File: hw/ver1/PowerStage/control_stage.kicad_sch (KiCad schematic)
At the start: 11 parts, among them J10 SWD Debug, J11 BMS_Serial, J8 FanConnector, P1 USB_C_Plug_USB2.0, SW2 I2C_Addr, U10 RP2040, U4 LM1117MP-3.3

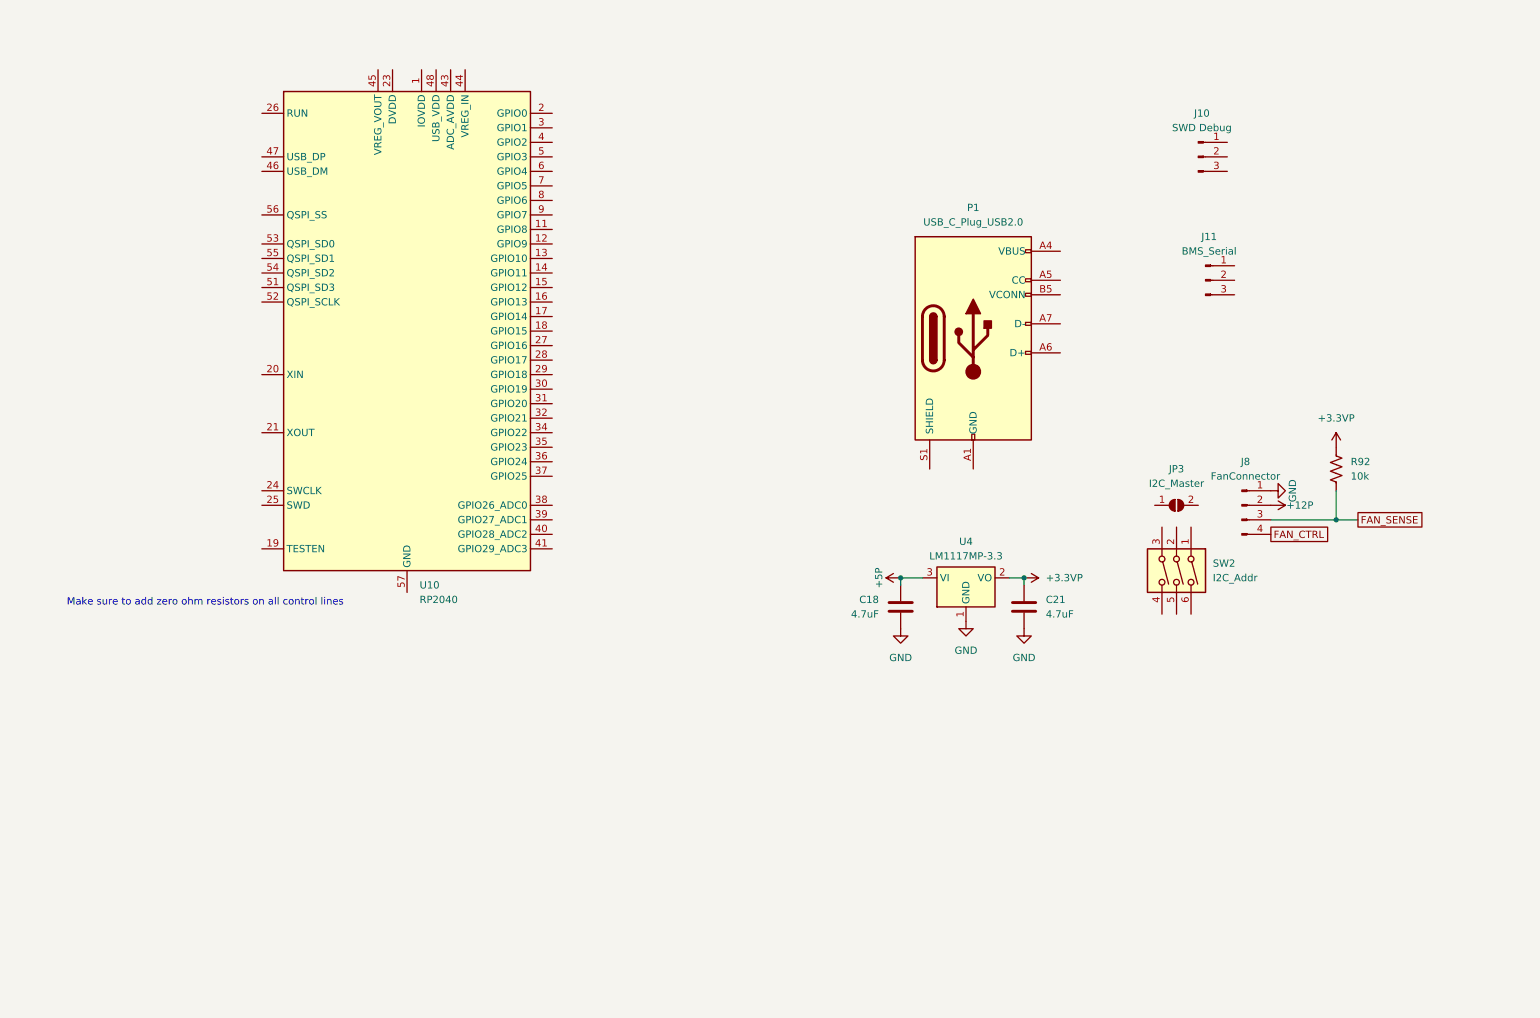
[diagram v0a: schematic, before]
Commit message: Sync this morning's effort
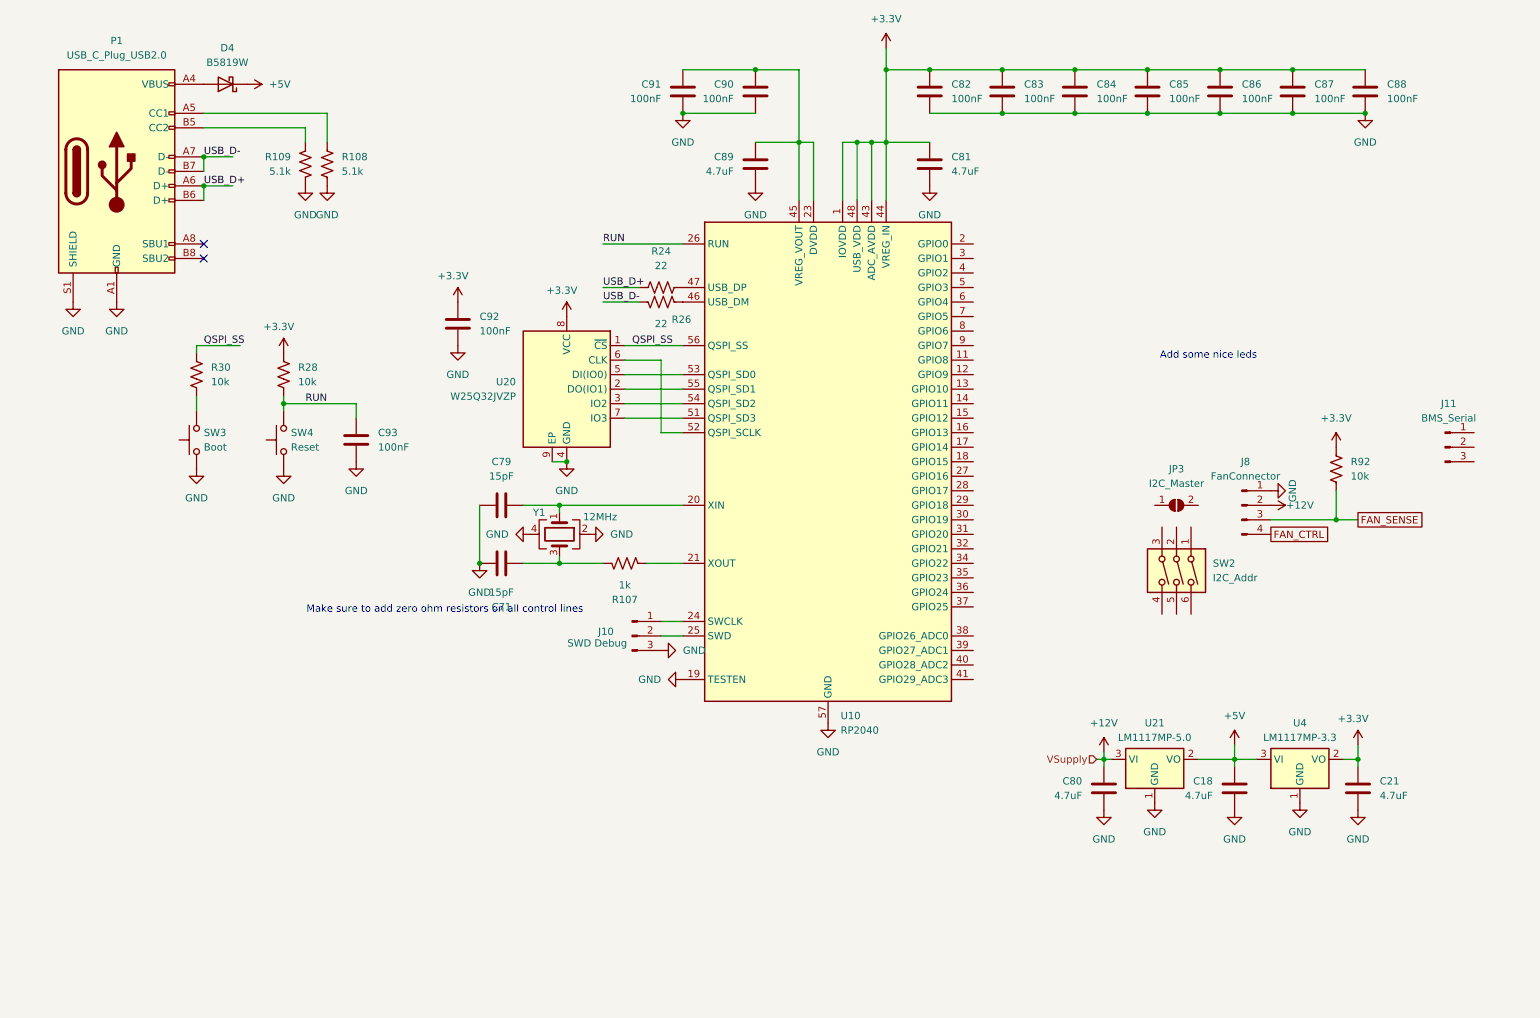
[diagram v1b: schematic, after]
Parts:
- added C71, C79: 15pF, Capacitor_SMD:C_0603_1608Metric, symbol Device:C
- added C80, C81, C89: 4.7uF, Capacitor_SMD:C_0603_1608Metric, symbol Device:C
- added C82, C83, C84, C85, C86, C87, C88, C90, C91, C92, C93: 100nF, Capacitor_SMD:C_0603_1608Metric, symbol Device:C
- added D4: B5819W, Diode_SMD:D_SOD-123, symbol Device:D_Schottky
- added R107: 1k, Resistor_SMD:R_0603_1608Metric, symbol Device:R_US
- added R108, R109: 5.1k, Resistor_SMD:R_0603_1608Metric, symbol Device:R_US
- added R24, R26: 22, Resistor_SMD:R_0603_1608Metric, symbol Device:R_US
- added R28, R30: 10k, Resistor_SMD:R_0603_1608Metric, symbol Device:R_US
- added SW3: Boot, symbol Switch:SW_Push
- added SW4: Reset, symbol Switch:SW_Push
- added U20: W25Q32JVZP, Package_SON:WSON-8-1EP_6x5mm_P1.27mm_EP3.4x4.3mm, symbol Memory_Flash:W25Q32JVZP
- added U21: LM1117MP-5.0, Package_TO_SOT_SMD:SOT-223-3_TabPin2, symbol Regulator_Linear:LM1117MP-5.0
- added Y1: 12MHz, Crystal:Crystal_SMD_3225-4Pin_3.2x2.5mm_HandSoldering, symbol Device:Crystal_GND24
- P1: symbol Connector:USB_C_Plug_USB2.0 -> Connector:USB_C_Receptacle_USB2.0_16P
- U4: LCSC C23984 -> C6186
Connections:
- net +3.3VP is gone; now on net +3.3V: C21.1, R92.2, U4.2 (VO)
- net GND: now also J10.3 (Pin_3), P1.A1 (GND), P1.A12 (GND), P1.B1 (GND), P1.B12 (GND), P1.S1 (SHIELD), U10.19 (TESTEN), U10.57 (GND), C71.1, C79.1, C80.2, C81.2, C82.2, C83.2, C84.2, C85.2, C86.2, C87.2, C88.2, C89.2, C90.2, C91.2, C92.2, C93.2, R108.1, R109.1, SW3.1, SW4.1, U20.4 (GND), U20.9 (EP), U21.1 (GND), Y1.2, Y1.4
- net +3.3V: now reaches U10.1 (IOVDD), U10.10 (IOVDD), U10.22 (IOVDD), U10.33 (IOVDD), U10.42 (IOVDD), U10.49 (IOVDD)
- net +3.3V: now also U10.43 (ADC_AVDD), U10.44 (VREG_IN), U10.48 (USB_VDD), C81.1, C82.1, C83.1, C84.1, C85.1, C86.1, C87.1, C88.1, C92.1, R28.2, U20.8 (VCC)
- net at U10.20 (XIN): now also C79.2, Y1.1
- net at U10.21 (XOUT): now also R107.2
- net at U10.23 (DVDD), U10.50 (DVDD): now also U10.45 (VREG_VOUT), C89.1, C90.1, C91.1
- net at U10.24 (SWCLK): now also J10.1 (Pin_1)
- net at U10.25 (SWD): now also J10.2 (Pin_2)
- net RUN: now reaches U10.26 (RUN)
- net RUN: now also C93.1, R28.1, SW4.2
- net at U10.46 (USB_DM): now also R26.1
- net at U10.47 (USB_DP): now also R24.1
- net at U10.51 (QSPI_SD3): now also U20.7 (IO3)
- net at U10.52 (QSPI_SCLK): now also U20.6 (CLK)
- net at U10.53 (QSPI_SD0): now also U20.5 (DI(IO0))
- net at U10.54 (QSPI_SD2): now also U20.3 (IO2)
- net at U10.55 (QSPI_SD1): now also U20.2 (DO(IO1))
- net QSPI_SS: now reaches U10.56 (QSPI_SS)
- net QSPI_SS: now also R30.2, U20.1 (~{CS})
- net at P1.A4 (VBUS), P1.A9 (VBUS), P1.B4 (VBUS)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: now also D4.2 (A)
- net at P1.A5 (CC1): now also R108.2
- net USB_D+: now reaches P1.A6 (D+)
- net USB_D+: now also P1.B6 (D+), R24.2
- net USB_D-: now reaches P1.A7 (D-)
- net USB_D-: now also P1.B7 (D-), R26.2
- net at P1.B5 (CC2): now also R109.2
- net +12P renamed +12V
- net +12V: now also C80.1, U21.3 (VI)
- net +5P renamed +5V
- net +5V: now also D4.1 (K), U21.2 (VO)
- new net: R30.1, SW3.2
- new net: C71.2, R107.1, Y1.3
- no-connect marks 0 -> 2
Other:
- note added: "Add some nice leds"
- moved on the sheet: C18, C21, J10, J11, U10, U4

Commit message: Sync tonight's effort
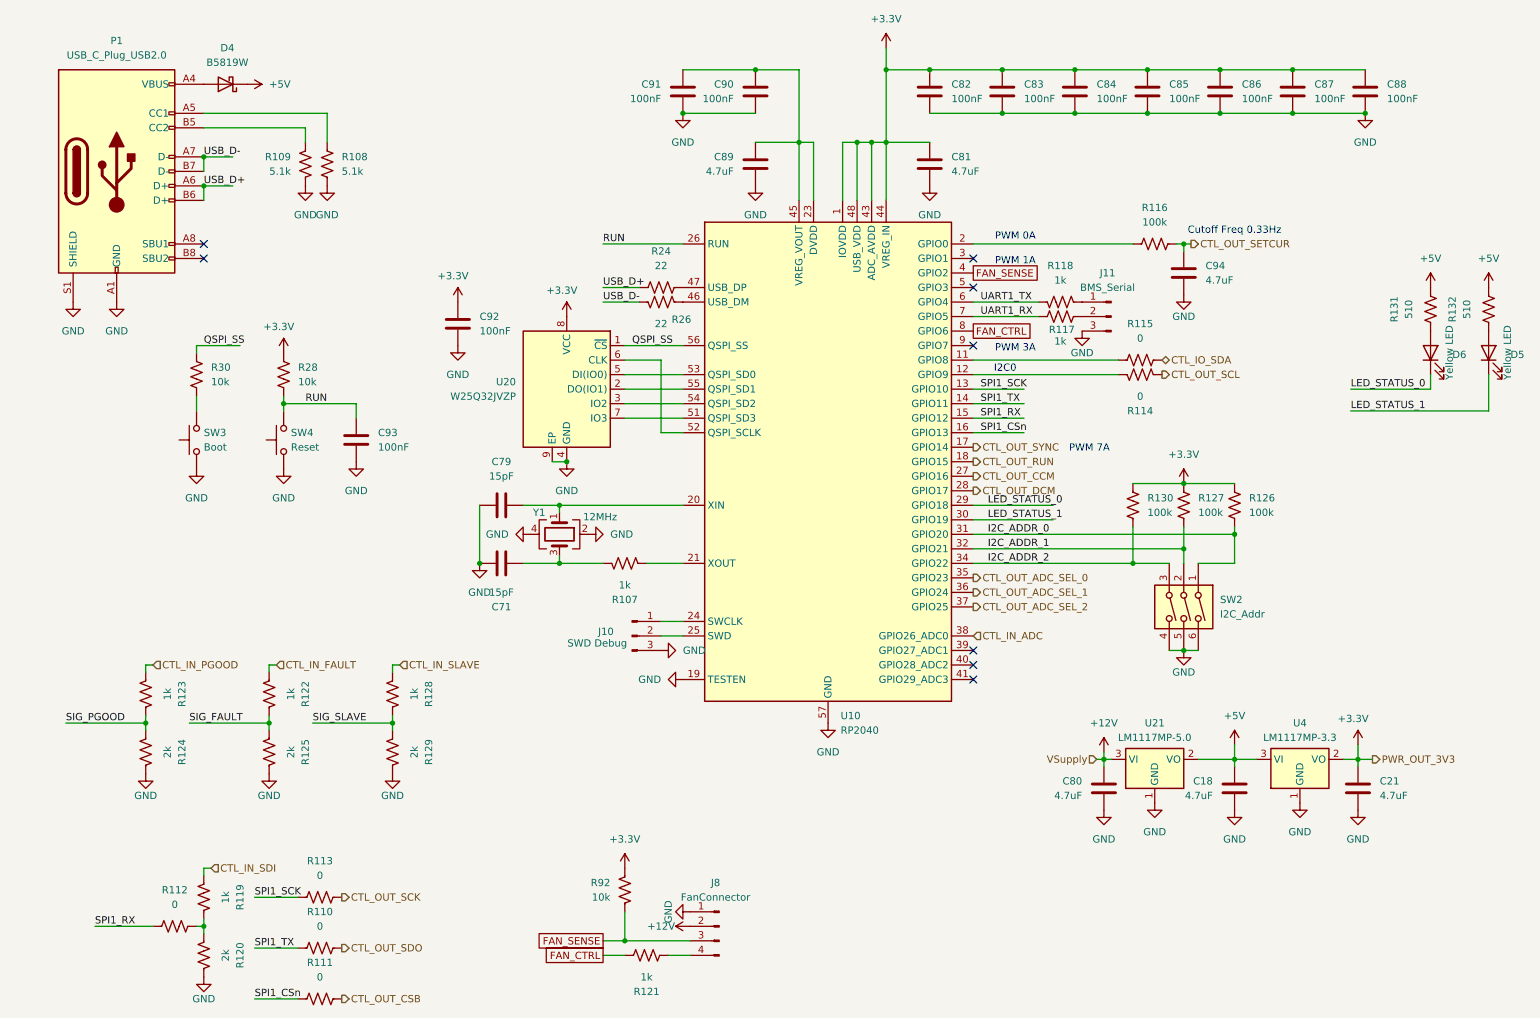
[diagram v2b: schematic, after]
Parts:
- removed JP3: I2C_Master, symbol Jumper:SolderJumper_2_Open
- added C94: 4.7uF, Capacitor_SMD:C_0603_1608Metric, symbol Device:C
- added D5, D6: Yellow LED, LED_SMD:LED_0805_2012Metric, symbol Device:LED
- added R110, R111, R112, R113, R114, R115: 0, Resistor_SMD:R_0603_1608Metric, symbol Device:R_US
- added R116, R126, R127, R130: 100k, Resistor_SMD:R_0603_1608Metric, symbol Device:R_US
- added R117, R118, R119, R121, R122, R123, R128: 1k, Resistor_SMD:R_0603_1608Metric, symbol Device:R_US
- added R120, R124, R125, R129: 2k, Resistor_SMD:R_0603_1608Metric, symbol Device:R_US
- added R131, R132: 510, Resistor_SMD:R_0603_1608Metric, symbol Device:R_US
- D4: Digikey (none) -> N/A
- J10, J11: Digikey (none) -> N/A; LCSC (none) -> N/A
- J8, P1, U20, Y1: LCSC (none) -> N/A
- SW3, SW4: footprint (none) -> Button_Switch_SMD:SW_SPST_EVQP2; Digikey (none) -> P11081SCT-ND; LCSC (none) -> N/A
- U10: Digikey (none) -> 2648-SC0914(13)CT-ND; LCSC (none) -> C2040
- U21: Digikey (none) -> N/A; LCSC (none) -> C6187
- U4: Digikey 488-LM1117MPX-33NOPBCT-ND -> N/A
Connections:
- net +3.3V: now also R126.2, R127.2, R130.2
- net +5V: now also R131.1, R132.1
- net FAN_CTRL: now also U10.8 (GPIO6), R121.2; no longer J8.4 (Pin_4)
- net FAN_SENSE: now also U10.4 (GPIO2)
- net GND: now also J11.3 (Pin_3), SW2.4, SW2.5, SW2.6, C94.2, R120.1, R124.1, R125.1, R129.1
- net at U10.11 (GPIO8): now also R115.2
- net at U10.12 (GPIO9): now also R114.2
- net SPI1_SCK: now reaches U10.13 (GPIO10)
- net SPI1_SCK: now also R113.2
- net SPI1_TX: now reaches U10.14 (GPIO11)
- net SPI1_TX: now also R110.2
- net SPI1_RX: now reaches U10.15 (GPIO12)
- net SPI1_RX: now also R112.2
- net SPI1_CSn: now reaches U10.16 (GPIO13)
- net SPI1_CSn: now also R111.2
- net CTL_OUT_SYNC: now reaches U10.17 (GPIO14)
- net CTL_OUT_RUN: now reaches U10.18 (GPIO15)
- net at U10.2 (GPIO0): now also R116.2
- net CTL_OUT_CCM: now reaches U10.27 (GPIO16)
- net CTL_OUT_DCM: now reaches U10.28 (GPIO17)
- net LED_STATUS_0: now reaches U10.29 (GPIO18)
- net LED_STATUS_0: now also D6.1 (K)
- net LED_STATUS_1: now reaches U10.30 (GPIO19)
- net LED_STATUS_1: now also D5.1 (K)
- net I2C_ADDR_0: now reaches U10.31 (GPIO20)
- net I2C_ADDR_0: now also SW2.1, R126.1
- net I2C_ADDR_1: now reaches U10.32 (GPIO21)
- net I2C_ADDR_1: now also SW2.2, R127.1
- net I2C_ADDR_2: now reaches U10.34 (GPIO22)
- net I2C_ADDR_2: now also SW2.3, R130.1
- net CTL_OUT_ADC_SEL_0: now reaches U10.35 (GPIO23)
- net CTL_OUT_ADC_SEL_1: now reaches U10.36 (GPIO24)
- net CTL_OUT_ADC_SEL_2: now reaches U10.37 (GPIO25)
- net CTL_IN_ADC: now reaches U10.38 (GPIO26_ADC0)
- net UART1_TX: now reaches U10.6 (GPIO4)
- net UART1_TX: now also R118.2
- net UART1_RX: now reaches U10.7 (GPIO5)
- net UART1_RX: now also R117.2
- net at J11.1 (Pin_1): now also R118.1
- net at J11.2 (Pin_2): now also R117.1
- new net: D6.2 (A), R131.2
- new net: J8.4 (Pin_4), R121.1
- new net: D5.2 (A), R132.2
- new net: R112.1, R119.1, R120.2
- new net CTL_IN_FAULT: R122.2
- new net CTL_IN_PGOOD: R123.2
- new net CTL_IN_SDI: R119.2
- new net CTL_IN_SLAVE: R128.2
- new net CTL_IO_SDA: R115.1
- new net CTL_OUT_CSB: R111.1
- new net CTL_OUT_SCK: R113.1
- new net CTL_OUT_SCL: R114.1
- new net CTL_OUT_SDO: R110.1
- new net CTL_OUT_SETCUR: C94.1, R116.1
- new net SIG_FAULT: R122.1, R125.2
- new net SIG_PGOOD: R123.1, R124.2
- new net SIG_SLAVE: R128.1, R129.2
- no-connect marks 2 -> 8
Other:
- note added: "Cutoff Freq 0.33Hz"
- note added: "I2C0"
- note added: "PWM 0A"
- note added: "PWM 1A"
- note added: "PWM 3A"
- note added: "PWM 7A"
- note removed: "Add some nice leds"
- note removed: "Make sure to add zero ohm resistors on all control lines"
- moved on the sheet: J11, J8, R92, SW2
